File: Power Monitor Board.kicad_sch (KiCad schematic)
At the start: 13 parts, among them U1 ACS709xLFTR-10BB, U10 ACS709xLFTR-10BB, U11 ACS709xLFTR-10BB, U12 ACS709xLFTR-10BB, U2 ACS709xLFTR-10BB, U3 ACS709xLFTR-10BB, U4 ACS709xLFTR-10BB, U5 ACS709xLFTR-10BB, U6 ACS709xLFTR-10BB, U7 ACS709xLFTR-10BB, U8 ACS709xLFTR-10BB, U9 ACS709xLFTR-10BB

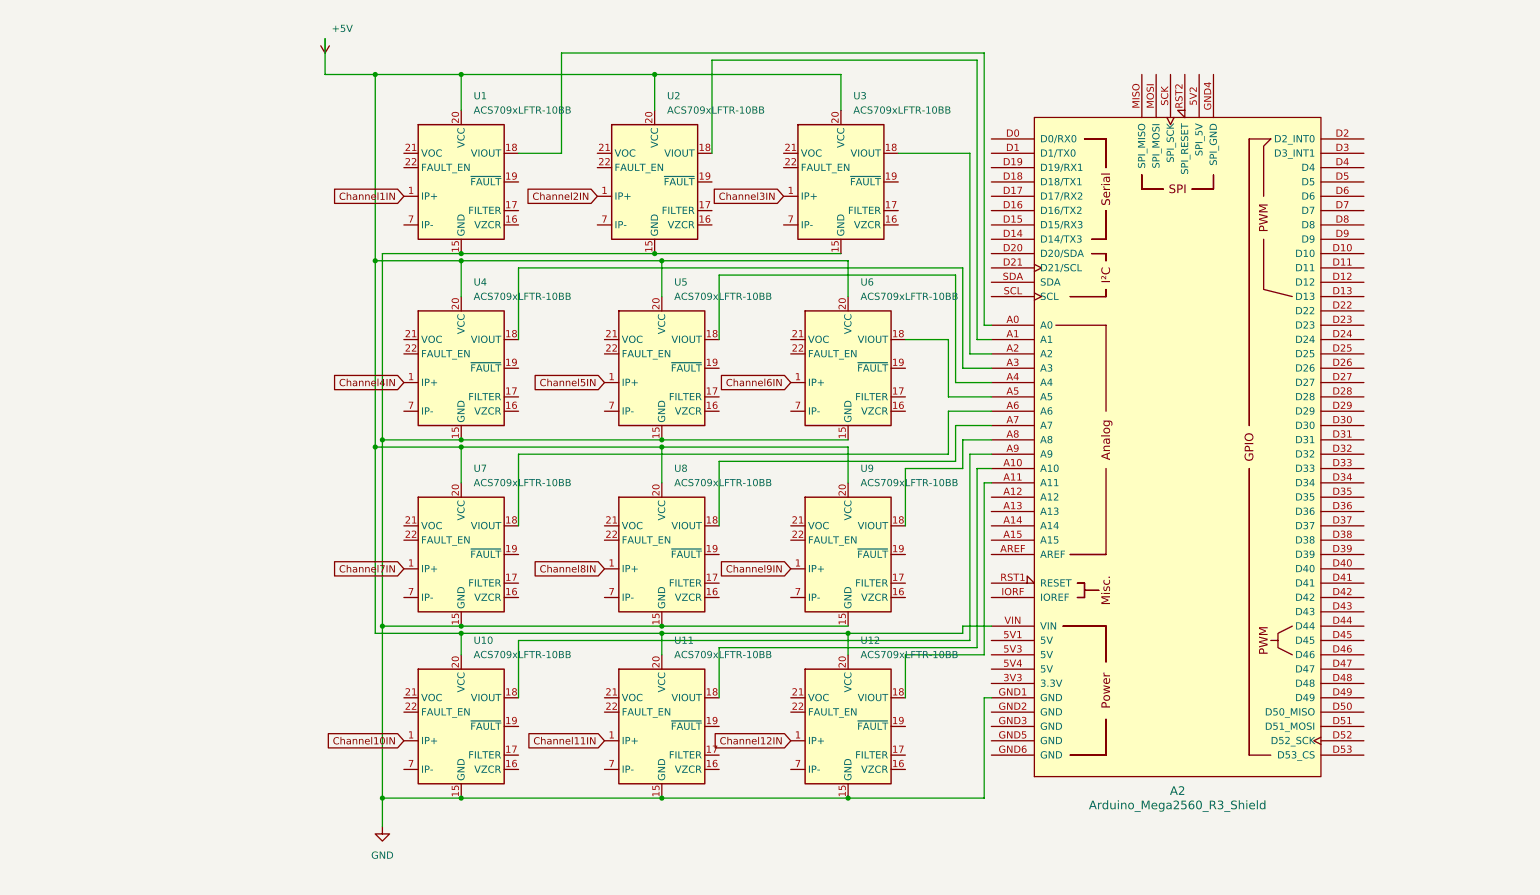
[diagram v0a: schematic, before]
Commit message: Add files via upload
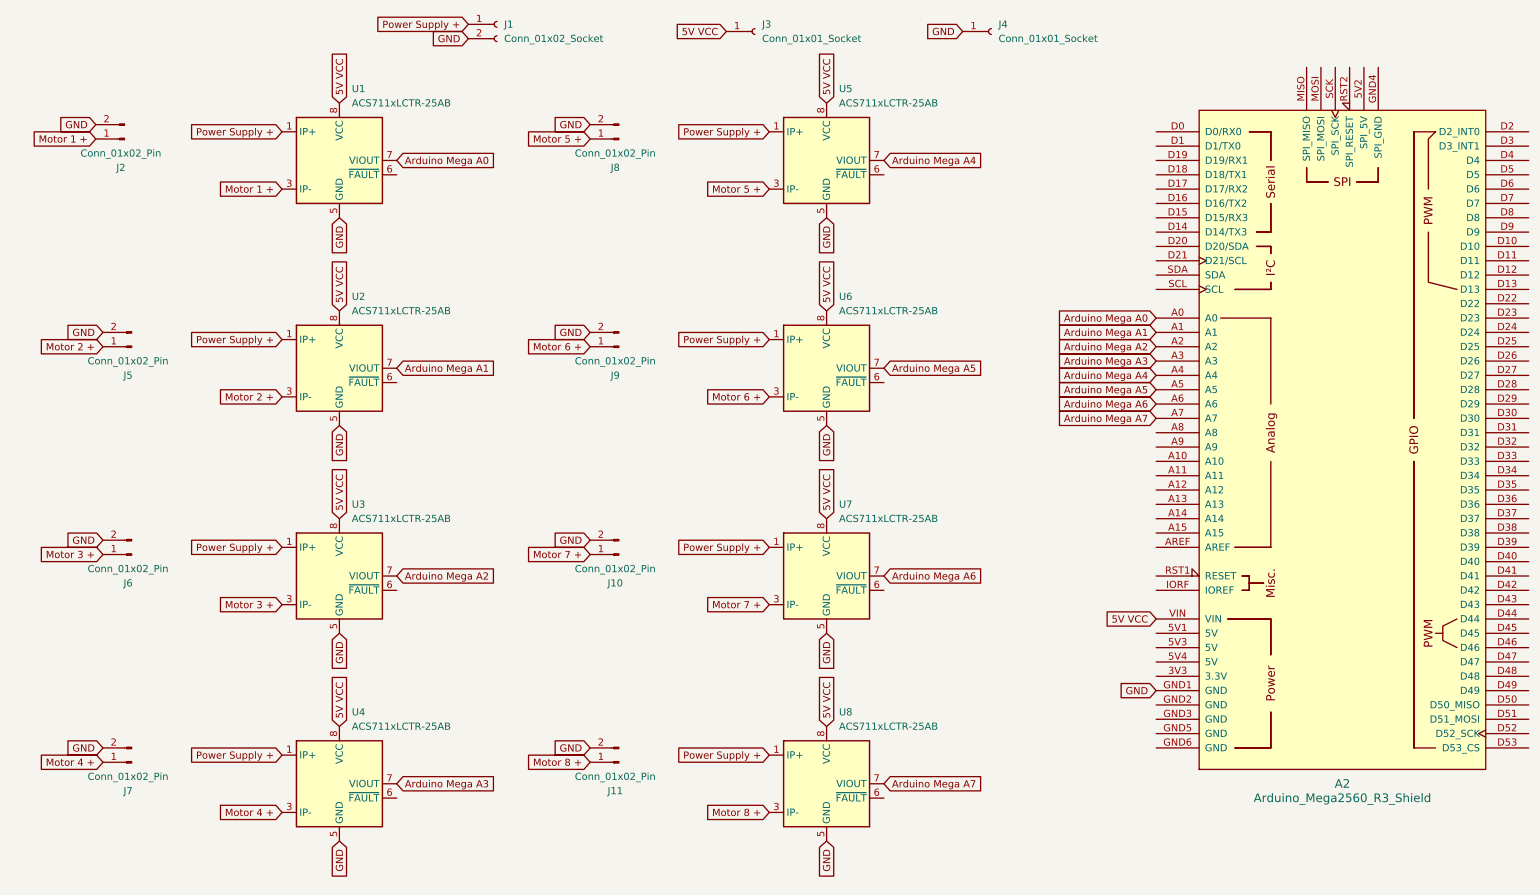
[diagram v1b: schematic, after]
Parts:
- removed U1, U10, U11, U12, U2, U3, U4, U5, U6, U7, U8, U9: ACS709xLFTR-10BB, Sensor_Current:Allegro_QSOP-24_3.9x8.7mm_P0.635mm, symbol Sensor_Current:ACS709xLFTR-10BB
- added J1: Conn_01x02_Socket, Connector:Banana_Jack_2Pin, symbol Connector:Conn_01x02_Socket
- added J10, J11, J2, J5, J6, J7, J8, J9: Conn_01x02_Pin, Connector_AMASS:AMASS_XT60-M_1x02_P7.20mm_Vertical, symbol Connector:Conn_01x02_Pin
- added J3, J4: Conn_01x01_Socket, Connector_PinSocket_2.54mm:PinSocket_1x01_P2.54mm_Vertical, symbol Connector:Conn_01x01_Socket
- added U1, U2, U3, U4, U5, U6, U7, U8: ACS711xLCTR-25AB, Package_SO:SOIC-8_3.9x4.9mm_P1.27mm, symbol Sensor_Current:ACS711xLCTR-25AB
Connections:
- net GND: now also J1.2 (Pin_2), J10.2 (Pin_2), J11.2 (Pin_2), J2.2 (Pin_2), J4.1 (Pin_1), J5.2 (Pin_2), J6.2 (Pin_2), J7.2 (Pin_2), J8.2 (Pin_2), J9.2 (Pin_2), U1.5 (GND), U2.5 (GND), U3.5 (GND), U4.5 (GND), U5.5 (GND), U6.5 (GND), U7.5 (GND), U8.5 (GND)
- net Arduino Mega A5: now reaches A2.A5
- net Arduino Mega A5: now also U6.7 (VIOUT)
- net Arduino Mega A1: now reaches A2.A1
- net Arduino Mega A1: now also U2.7 (VIOUT)
- net Arduino Mega A2: now reaches A2.A2
- net Arduino Mega A2: now also U3.7 (VIOUT)
- net Arduino Mega A4: now reaches A2.A4
- net Arduino Mega A4: now also U5.7 (VIOUT)
- net Arduino Mega A7: now reaches A2.A7
- net Arduino Mega A7: now also U8.7 (VIOUT)
- net Arduino Mega A6: now reaches A2.A6
- net Arduino Mega A6: now also U7.7 (VIOUT)
- net Arduino Mega A0: now reaches A2.A0
- net Arduino Mega A0: now also U1.7 (VIOUT)
- net Arduino Mega A3: now reaches A2.A3
- net Arduino Mega A3: now also U4.7 (VIOUT)
- net +5V renamed 5V VCC
- net 5V VCC: now also J3.1 (Pin_1), U1.8 (VCC), U2.8 (VCC), U3.8 (VCC), U4.8 (VCC), U5.8 (VCC), U6.8 (VCC), U7.8 (VCC), U8.8 (VCC)
- new net Motor 1 +: J2.1 (Pin_1), U1.3 (IP-), U1.4 (IP-)
- new net Motor 2 +: J5.1 (Pin_1), U2.3 (IP-), U2.4 (IP-)
- new net Motor 3 +: J6.1 (Pin_1), U3.3 (IP-), U3.4 (IP-)
- new net Motor 4 +: J7.1 (Pin_1), U4.3 (IP-), U4.4 (IP-)
- new net Motor 5 +: J8.1 (Pin_1), U5.3 (IP-), U5.4 (IP-)
- new net Motor 6 +: J9.1 (Pin_1), U6.3 (IP-), U6.4 (IP-)
- new net Motor 7 +: J10.1 (Pin_1), U7.3 (IP-), U7.4 (IP-)
- new net Motor 8 +: J11.1 (Pin_1), U8.3 (IP-), U8.4 (IP-)
- new net Power Supply +: J1.1 (Pin_1), U1.1 (IP+), U1.2 (IP+), U2.1 (IP+), U2.2 (IP+), U3.1 (IP+), U3.2 (IP+), U4.1 (IP+), U4.2 (IP+), U5.1 (IP+), U5.2 (IP+), U6.1 (IP+), U6.2 (IP+), U7.1 (IP+), U7.2 (IP+), U8.1 (IP+), U8.2 (IP+)
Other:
- moved on the sheet: A2
